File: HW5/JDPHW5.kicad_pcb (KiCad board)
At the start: 2 copper layers, 16 parts, among them J1 Conn_01x03_Pin, J2 Conn_01x02_Pin, U1 NSL-32, U2 NSL-32, U3 TLV2372

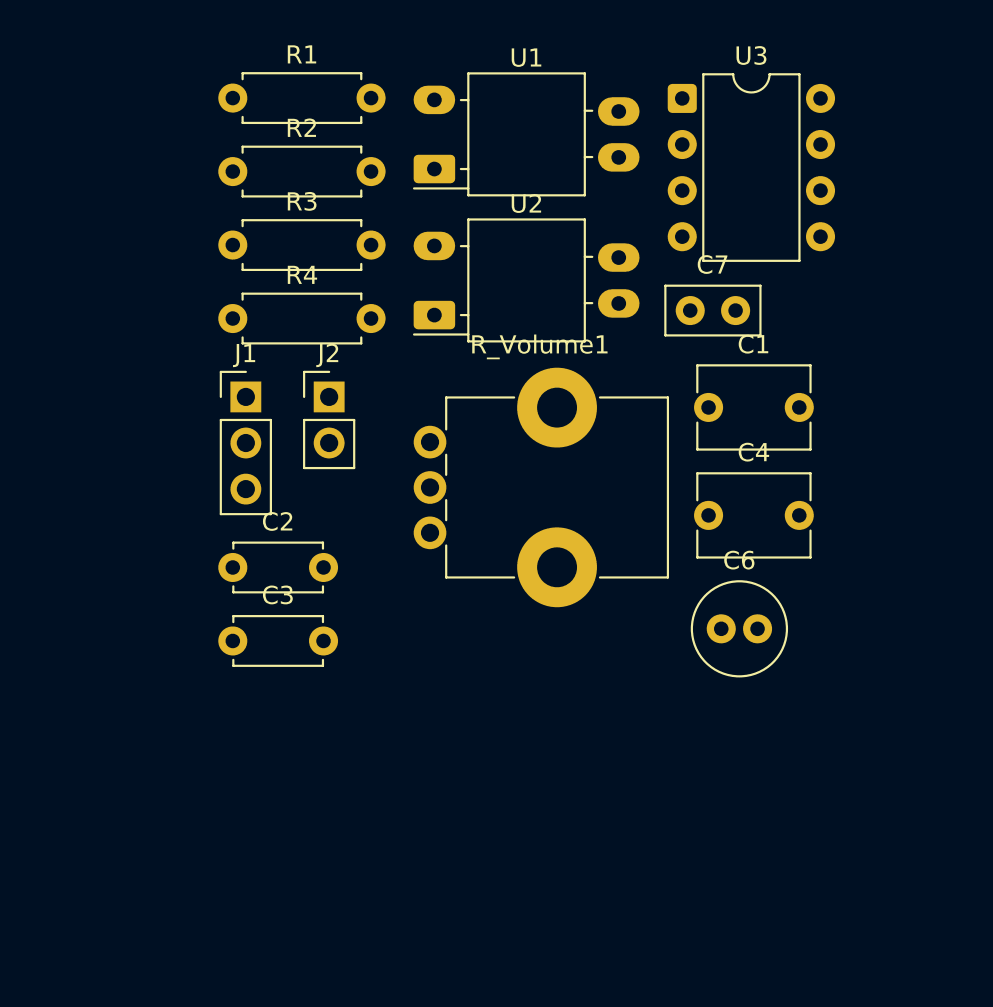
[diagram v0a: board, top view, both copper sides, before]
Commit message: Final
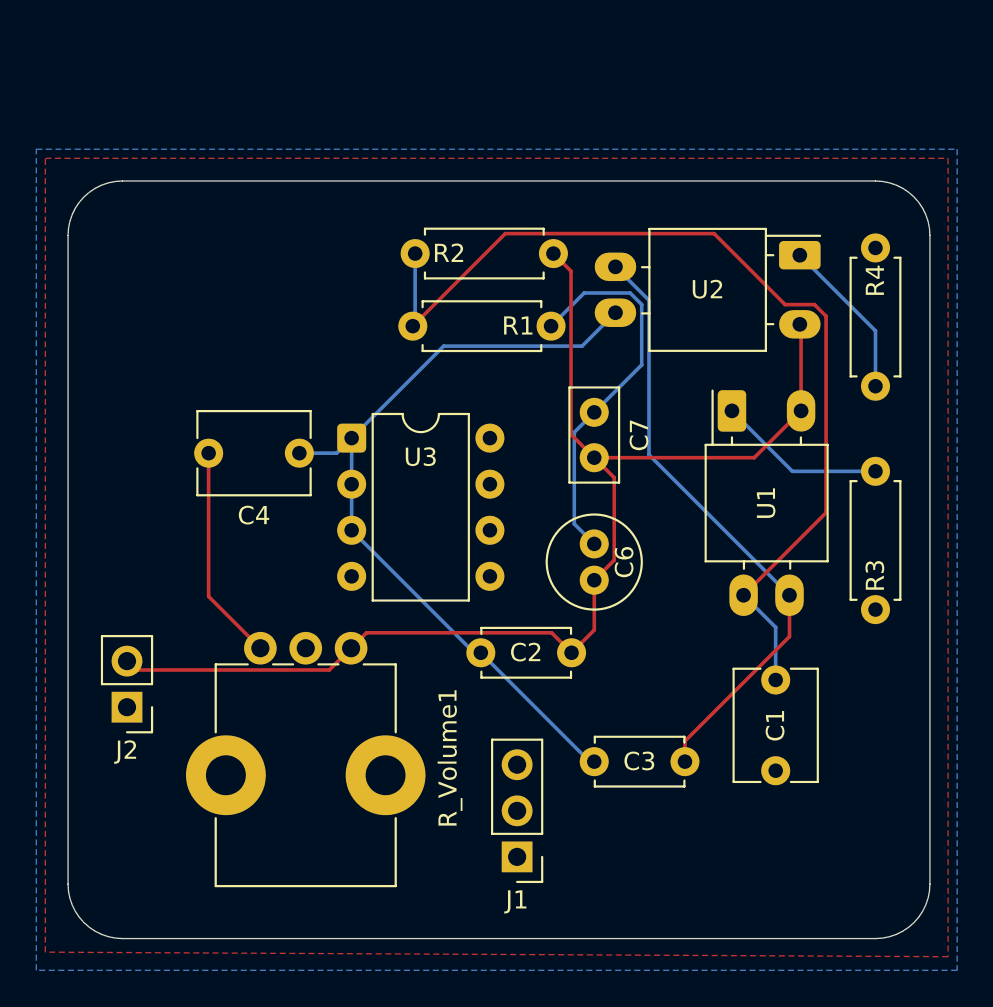
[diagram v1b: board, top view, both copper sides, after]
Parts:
- moved R3 40.7 mm to (157.2, 103.6), turned to 90 degrees
- moved R4 35.6 mm to (157.2, 83.7), turned to -90 degrees
- moved J1 29.4 mm to (137.5, 117.2), turned to 180 degrees
- moved U3 26.1 mm to (128.4, 94.2)
- moved C3 25.8 mm to (146.8, 112.0), turned to 180 degrees
- moved C4 22.8 mm to (125.5, 95.0), turned to 180 degrees
- moved R1 21.6 mm to (139.4, 88.0), turned to 180 degrees
- moved U1 21.1 mm to (149.3, 92.7), turned to -90 degrees
- moved U2 20.4 mm to (153.1, 84.1), turned to 180 degrees
- moved J2 20.4 mm to (116.0, 109.0), turned to 180 degrees
- moved C1 20.4 mm to (151.8, 112.5), turned to 90 degrees
- moved C2 14.5 mm to (135.5, 106.0)
- moved R_Volume1 11.3 mm to (123.3, 105.8), turned to -90 degrees
- moved R2 11.0 mm to (131.9, 84.0)
- moved C6 8.42 mm to (141.8, 100.0), turned to -90 degrees
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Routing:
- net GND: track 0.00 -> 67.6 mm
- net Net-(C1-Pad2): track 0.00 -> 53.5 mm
- net Net-(U3A-+): track 0.00 -> 44.4 mm
- net Net-(C3-Pad1): track 0.00 -> 33.6 mm
- net VCC: track 0.00 -> 21.2 mm
- net Net-(C4-Pad2): track 0.00 -> 12.3 mm
- net Net-(U1-A): track 0.00 -> 9.29 mm
- net Net-(U2-A): track 0.00 -> 8.95 mm
- added copper zone on F.Cu, net GND
- added copper zone on B.Cu, net VCC
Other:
- board outline added: 47.5 x 41.8 mm
